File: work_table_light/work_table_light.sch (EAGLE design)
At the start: 32 parts, among them IC1 TINY24/44/84-PU, Q1 IRFP250, Q4 IRFP250, Q6 IRFP250, Q7 IRFP250

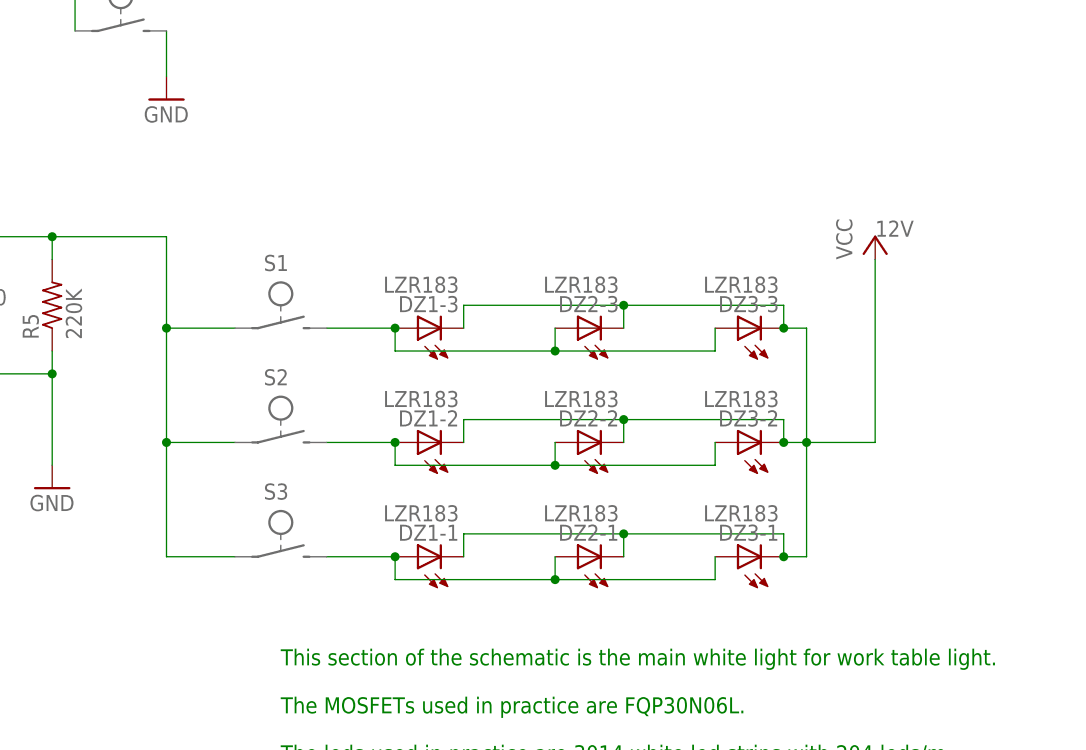
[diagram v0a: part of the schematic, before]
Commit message: updated schematic
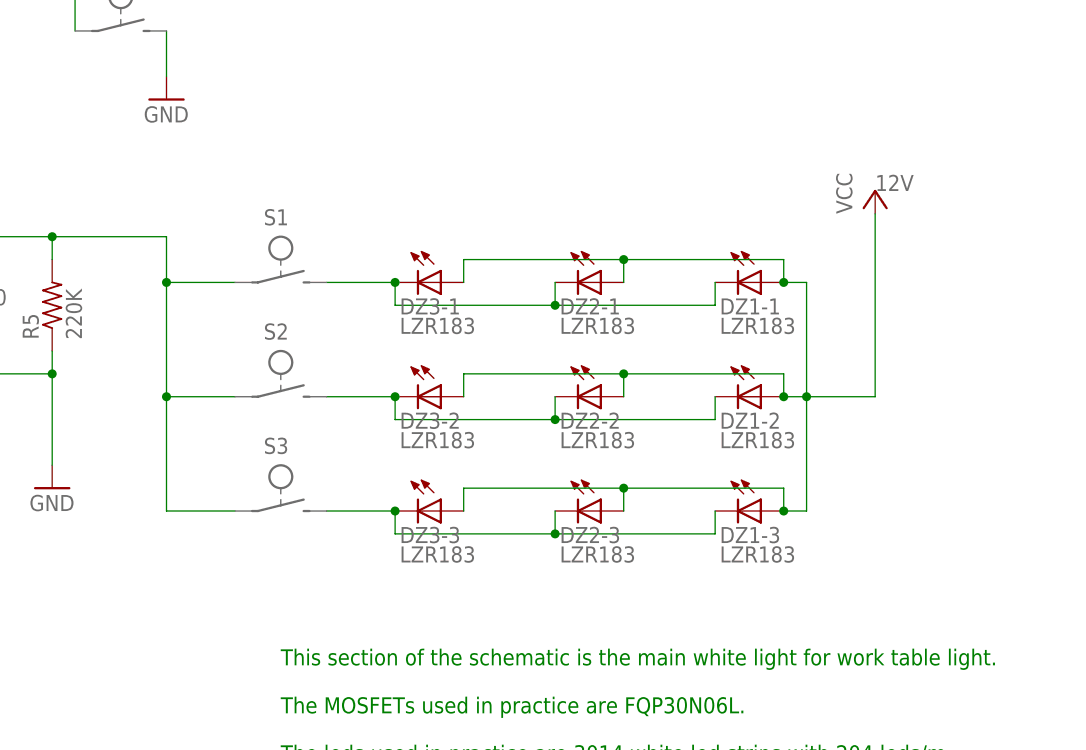
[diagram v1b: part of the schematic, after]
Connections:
- removed net N$4: DZ1-2.A, DZ2-2.A, DZ3-2.A
- removed net N$5: DZ1-1.A, DZ2-1.A, DZ3-1.A
- new net N$12: DZ1-1.C, DZ2-1.C, DZ3-1.C
- new net N$13: DZ1-2.C, DZ2-2.C, DZ3-2.C
- net N$2: now also DZ1-3.C, DZ2-3.C, DZ3-3.C; no longer DZ1-3.A, DZ2-3.A, DZ3-3.A
- net VCC: now also DZ1-1.A, DZ1-2.A, DZ1-3.A, DZ2-1.A, DZ2-2.A, DZ2-3.A, DZ3-1.A, DZ3-2.A, DZ3-3.A; no longer DZ1-1.C, DZ1-2.C, DZ1-3.C, DZ2-1.C, DZ2-2.C, DZ2-3.C, DZ3-1.C, DZ3-2.C, DZ3-3.C
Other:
- moved on the sheet: DZ1-1, DZ1-2, DZ1-3, DZ2-1, DZ2-2, DZ2-3, DZ3-1, DZ3-2, DZ3-3, S1, S2, S3
